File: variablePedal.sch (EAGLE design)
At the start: 16 parts, among them IC1 OPA340U, J2 AUDIO_JACK_TRS_0.25"_PTH_RA, J3 AUDIO_JACK_TRS_0.25"_PTH_RA, J4 5.5x2.1mm Barrel, Q1 MPSA56

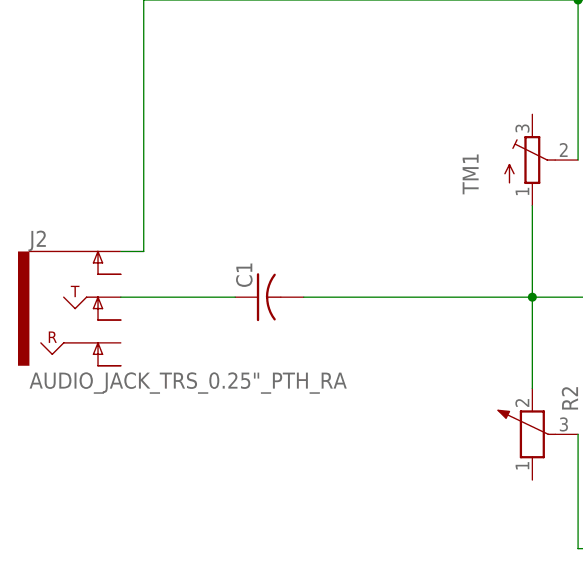
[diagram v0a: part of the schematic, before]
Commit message: Some finishing touches (labels, tidy placement)
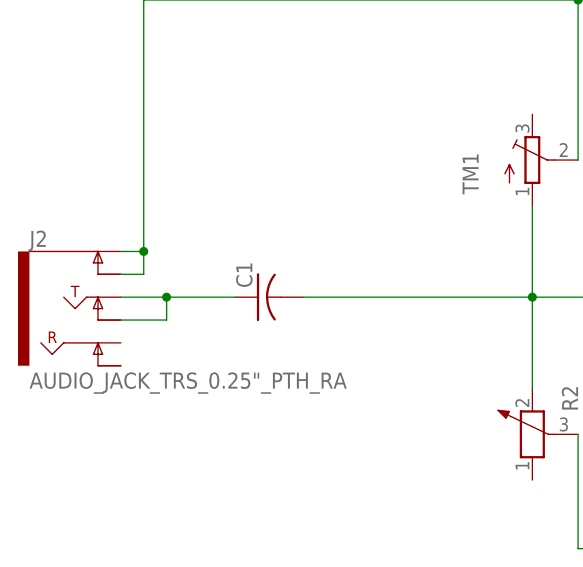
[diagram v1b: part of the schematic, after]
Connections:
- net GND: now also J2.EARTH-NORM
- net N$11: now also J2.TIP-NORM
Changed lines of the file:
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@@
 <wire x1="20.32" y1="99.06" x2="68.58" y2="99.06" width="0.1524" layer="91"/>
 <junction x="68.58" y="99.06"/>
+<pinref part="J2" gate="G$1" pin="EARTH-NORM"/>
+<wire x1="17.78" y1="68.58" x2="20.32" y2="68.58" width="0.1524" layer="91"/>
+<wire x1="20.32" y1="68.58" x2="20.32" y2="71.12" width="0.1524" layer="91"/>
+<junction x="20.32" y="71.12"/>
 </segment>
 </net>
@@
 <pinref part="J2" gate="G$1" pin="TIP"/>
 <pinref part="C1" gate="G$1" pin="1"/>
-<wire x1="17.78" y1="66.04" x2="30.48" y2="66.04" width="0.1524" layer="91"/>
+<wire x1="17.78" y1="66.04" x2="22.86" y2="66.04" width="0.1524" layer="91"/>
+<pinref part="J2" gate="G$1" pin="TIP-NORM"/>
+<wire x1="22.86" y1="66.04" x2="30.48" y2="66.04" width="0.1524" layer="91"/>
+<wire x1="17.78" y1="63.5" x2="22.86" y2="63.5" width="0.1524" layer="91"/>
+<wire x1="22.86" y1="63.5" x2="22.86" y2="66.04" width="0.1524" layer="91"/>
+<junction x="22.86" y="66.04"/>
 </segment>
 </net>

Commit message: Revert "Some finishing touches (labels, tidy placement)"
This reverts commit a6e963cb4720da940ed62cc4250a87c95adb02c4.
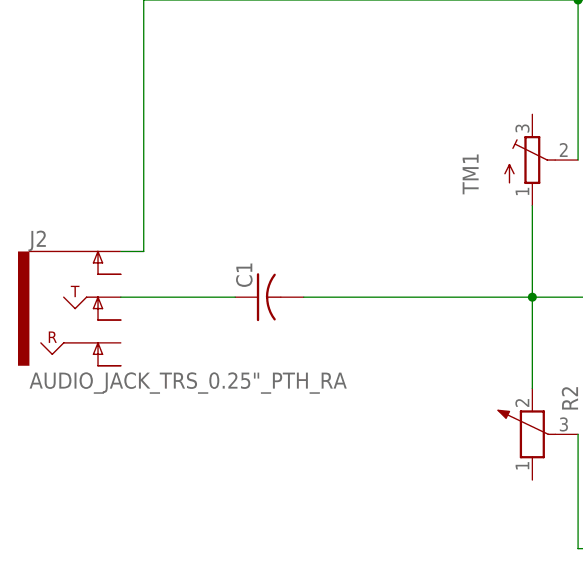
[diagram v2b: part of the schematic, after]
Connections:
- net GND: no longer J2.EARTH-NORM
- net N$11: no longer J2.TIP-NORM
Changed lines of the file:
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@@
 <wire x1="20.32" y1="99.06" x2="68.58" y2="99.06" width="0.1524" layer="91"/>
 <junction x="68.58" y="99.06"/>
-<pinref part="J2" gate="G$1" pin="EARTH-NORM"/>
-<wire x1="17.78" y1="68.58" x2="20.32" y2="68.58" width="0.1524" layer="91"/>
-<wire x1="20.32" y1="68.58" x2="20.32" y2="71.12" width="0.1524" layer="91"/>
-<junction x="20.32" y="71.12"/>
 </segment>
 </net>
@@
 <pinref part="J2" gate="G$1" pin="TIP"/>
 <pinref part="C1" gate="G$1" pin="1"/>
-<wire x1="17.78" y1="66.04" x2="22.86" y2="66.04" width="0.1524" layer="91"/>
-<pinref part="J2" gate="G$1" pin="TIP-NORM"/>
-<wire x1="22.86" y1="66.04" x2="30.48" y2="66.04" width="0.1524" layer="91"/>
-<wire x1="17.78" y1="63.5" x2="22.86" y2="63.5" width="0.1524" layer="91"/>
-<wire x1="22.86" y1="63.5" x2="22.86" y2="66.04" width="0.1524" layer="91"/>
-<junction x="22.86" y="66.04"/>
+<wire x1="17.78" y1="66.04" x2="30.48" y2="66.04" width="0.1524" layer="91"/>
 </segment>
 </net>
